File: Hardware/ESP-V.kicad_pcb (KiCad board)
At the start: 2 copper layers, 29.1 x 48.2 mm, 53 parts, among them J1 USB_C_Receptacle_USB2.0, J2 Conn_01x16_Male, J3 Conn_01x14_Female, J4 Conn_Coaxial, U1 AT25xxx-MA, U2 AP7333-33SRG-7, U3 AP7333-33SRG-7, U4 ESP32-C3, U5 CH552G, Y1 40MHz, Y2 32k

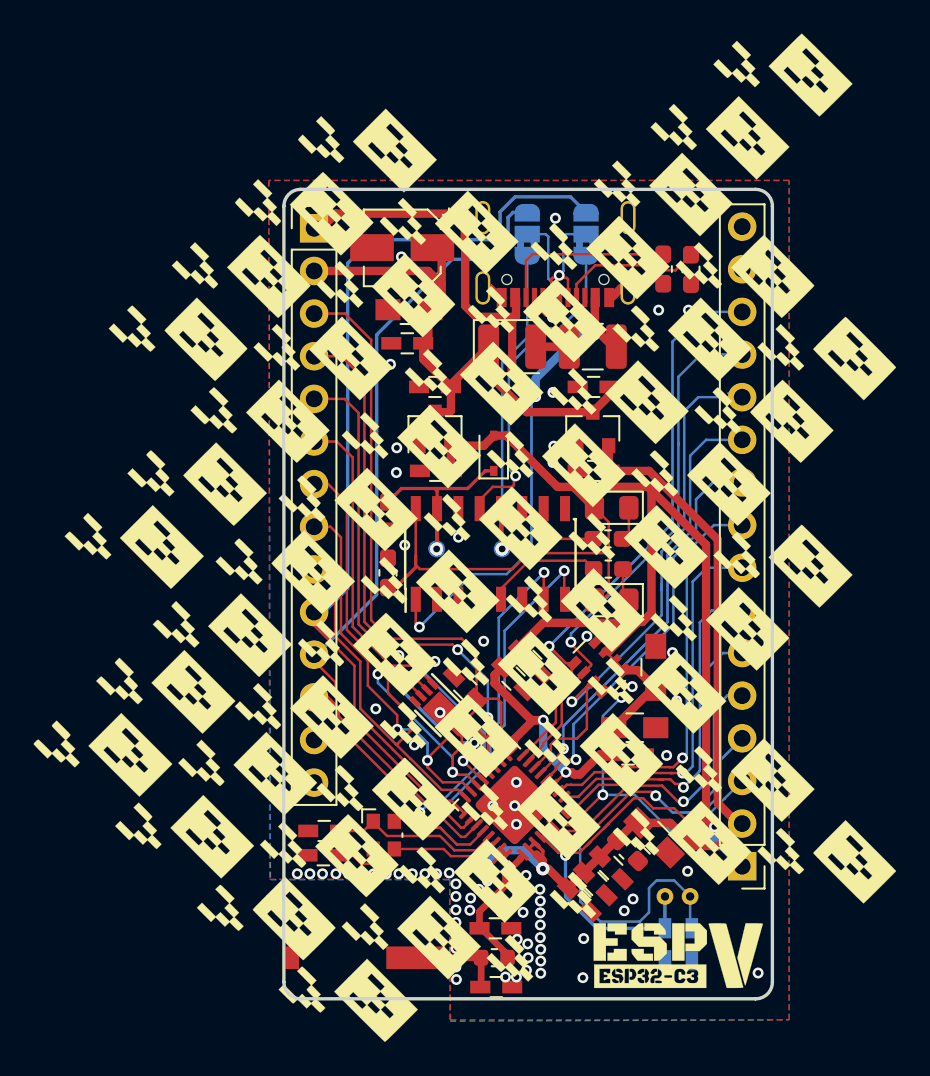
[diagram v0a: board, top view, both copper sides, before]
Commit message: ready to order needs final check
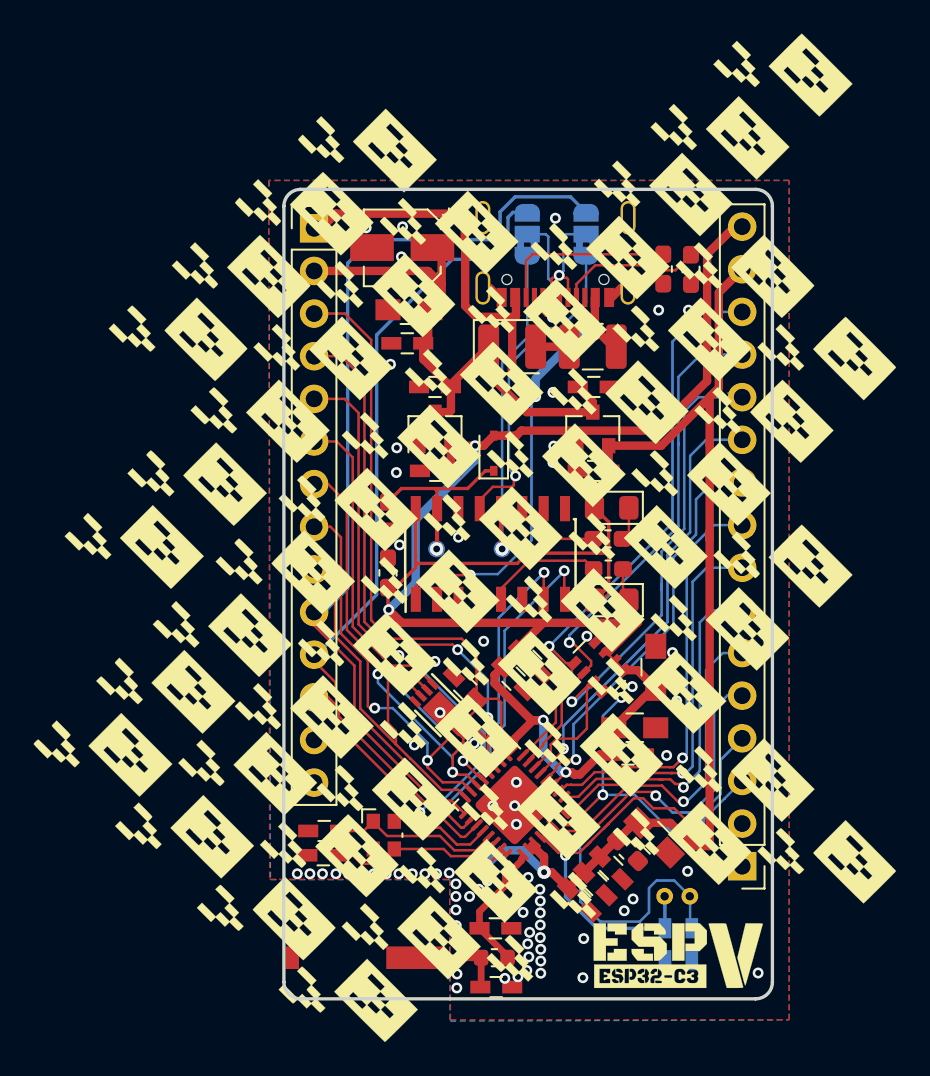
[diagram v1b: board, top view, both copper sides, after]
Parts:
- added G***: LOGO, art and silk:backsilk, B.Cu at (102.3, 100.8)
- Y2: footprint Crystal:Crystal_DS10_D1.0mm_L4.3mm_Horizontal -> footprint:Crystal_DS10_D1.0mm_L4.3mm_Horizontalnosilk
- turned C5 to 0 degrees
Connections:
- J2 pad 1: +3V3 -> GND
- J2 pad 15: GND -> +3.3VA
- J2 pad 16: GND -> +3V3
- J2 pad 2: +3.3VA -> GND
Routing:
- net +3.3VA: track 52.2 -> 66.0 mm
- net +3V3: track 117.7 -> 124.3 mm, vias 3 -> 4
- net VBUS: track 53.8 -> 51.7 mm
- net /GP17: track 26.1 -> 25.3 mm
- net GND: track 3.02 -> 3.57 mm, vias 81 -> 80
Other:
- board text added: "V1.0"
